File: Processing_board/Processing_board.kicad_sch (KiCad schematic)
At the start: 28 parts, among them J1 Conn_01x08_Pin, J2 Conn_01x08_Pin, J3 Conn_01x06_Pin, J4 Conn_01x03_Pin, J5 Conn_01x03_Pin, J6 Conn_01x02_Pin, J7 Conn_01x02_Pin, SW1 TL3305BF100QG, SW2 TL3305BF100QG, U1 STM32WBA63CIU6

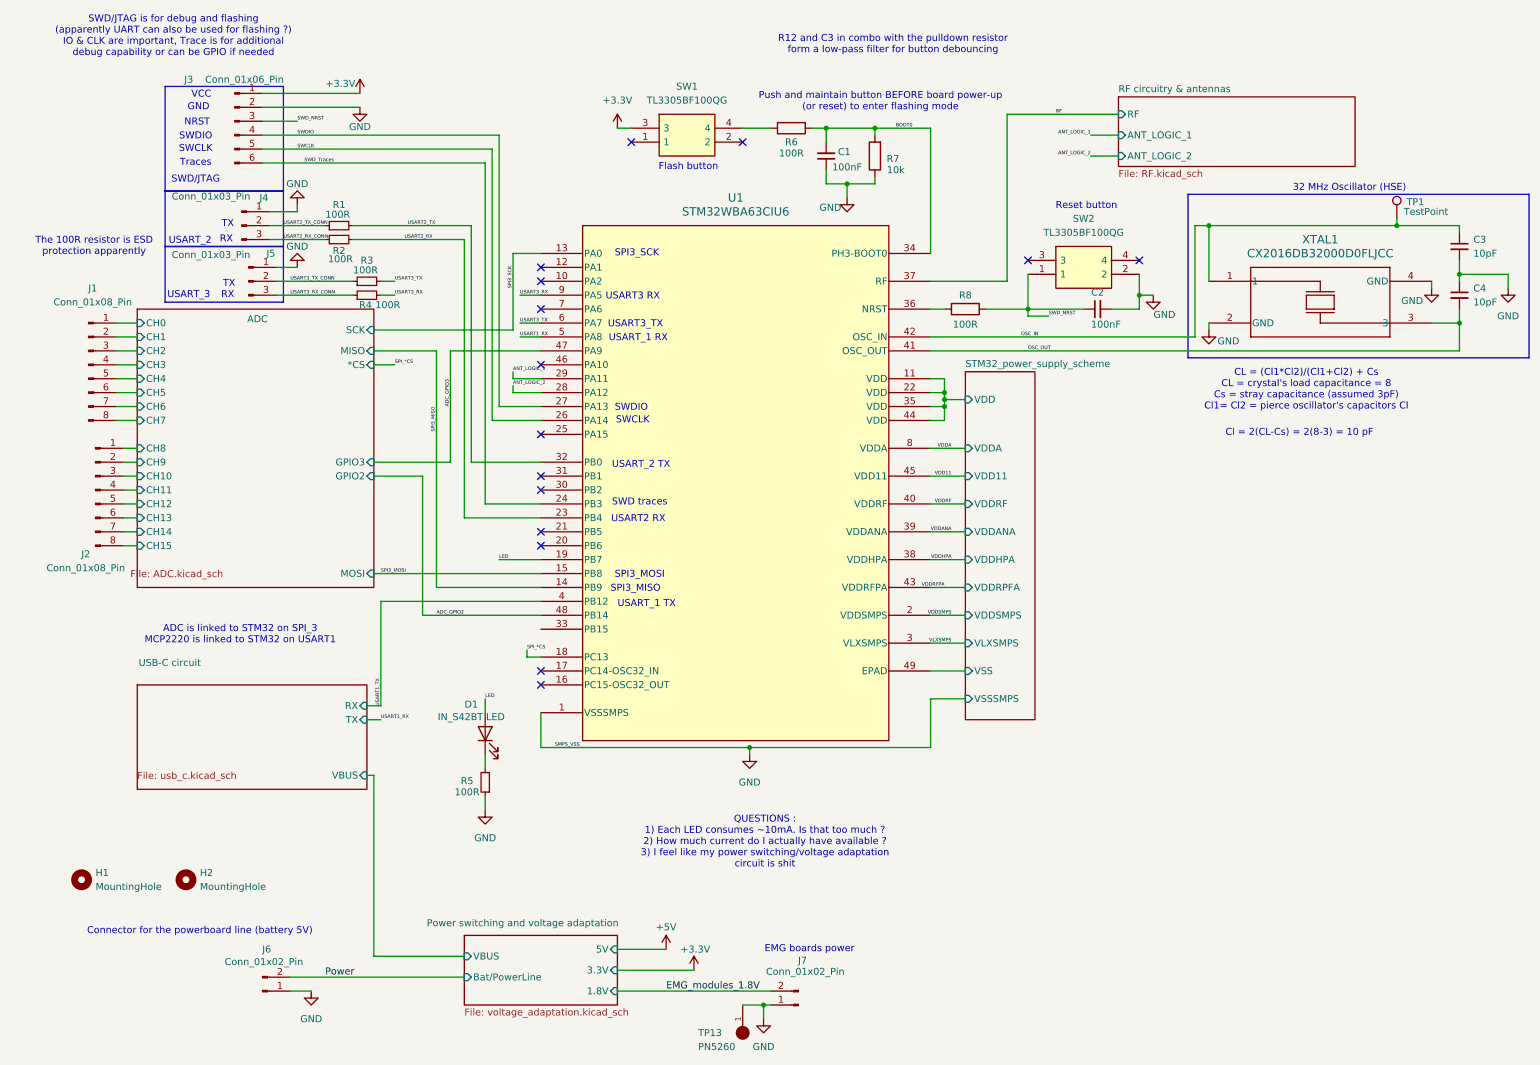
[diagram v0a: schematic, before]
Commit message: more cleanup
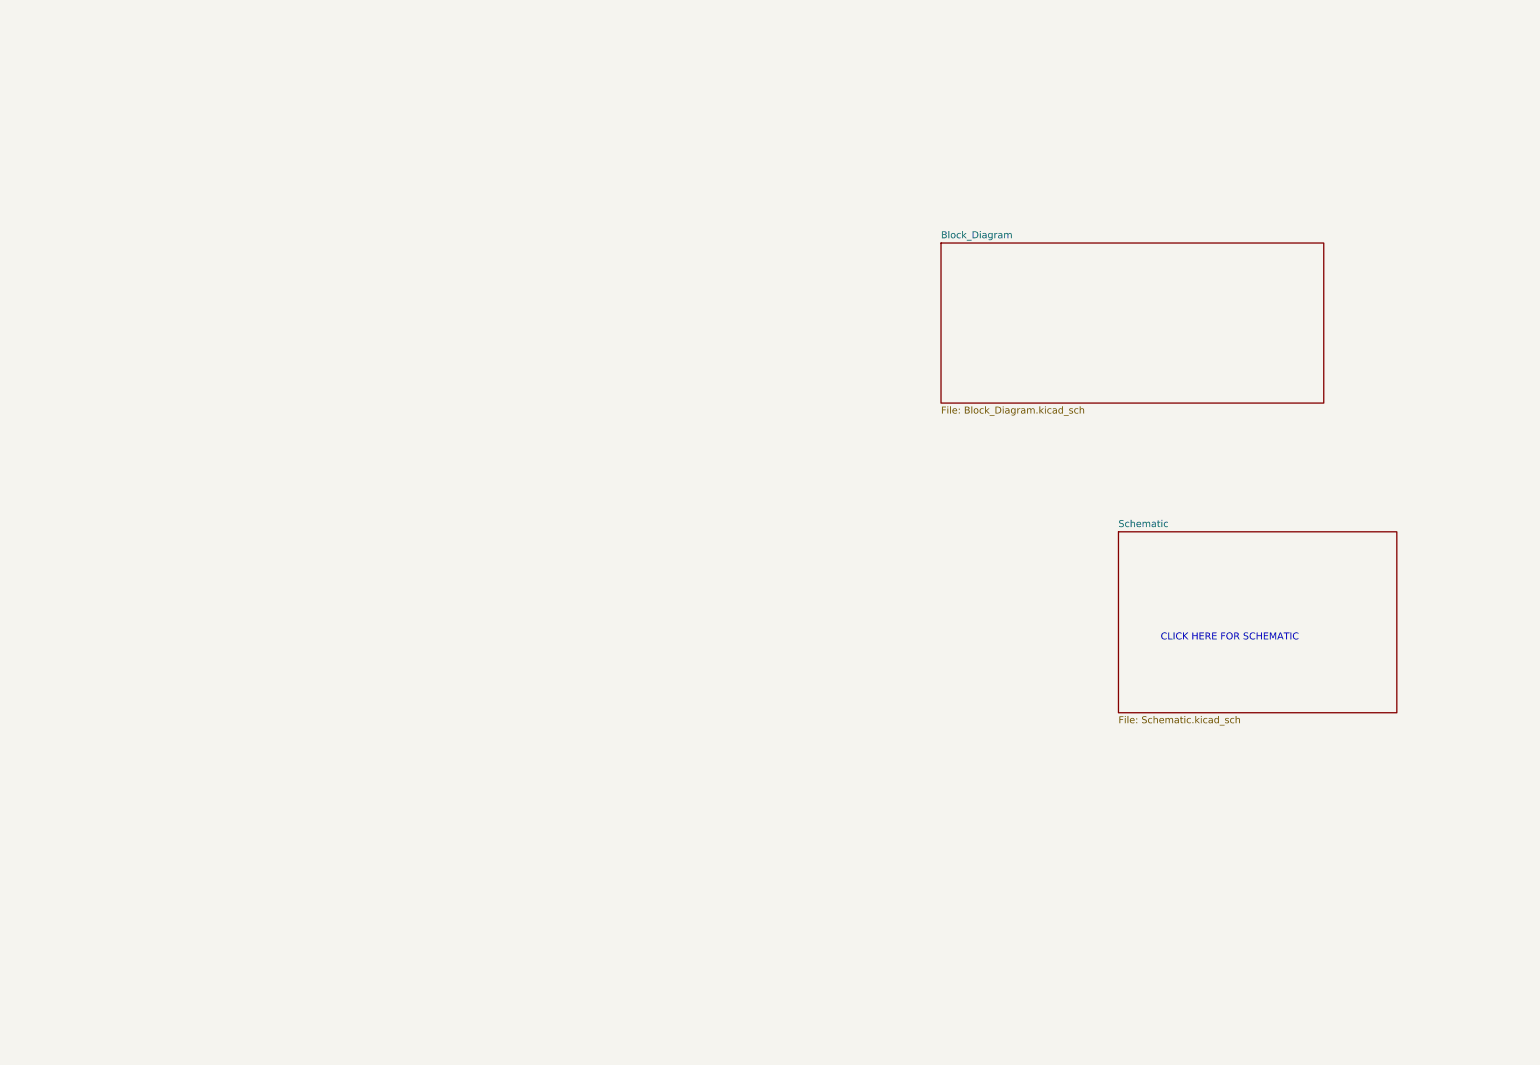
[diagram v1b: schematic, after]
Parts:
- removed C1, C2: 100nF, Capacitor_SMD:C_0402_1005Metric, symbol Device:C_Small
- removed C3, C4: 10pF, Capacitor_SMD:C_0603_1608Metric, symbol Device:C_Small
- removed D1: IN_S42BT LED, LED_SMD:LED_0402_1005Metric, symbol Device:LED
- removed H1, H2: MountingHole, MountingHole:MountingHole_2.2mm_M2, symbol Mechanical:MountingHole
- removed J1, J2: Conn_01x08_Pin, Connector_PinHeader_2.54mm:PinHeader_1x08_P2.54mm_Vertical_SMD_Pin1Left, symbol Connector:Conn_01x08_Pin
- removed J3: Conn_01x06_Pin, Connector_PinHeader_2.54mm:PinHeader_1x06_P2.54mm_Vertical_SMD_Pin1Left, symbol Connector:Conn_01x06_Pin
- removed J4, J5: Conn_01x03_Pin, Connector_PinHeader_2.54mm:PinHeader_1x03_P2.54mm_Vertical_SMD_Pin1Left, symbol Connector:Conn_01x03_Pin
- removed J6, J7: Conn_01x02_Pin, Connector_PinHeader_2.54mm:PinHeader_1x02_P2.54mm_Vertical_SMD_Pin1Left, symbol Connector:Conn_01x02_Pin
- removed R1, R2, R3, R4, R5: 100R, Resistor_SMD:R_0402_1005Metric, symbol Device:R_Small
- removed R6, R8: 100R, Resistor_SMD:R_0402_1005Metric, symbol Device:R
- removed R7: 10k, Resistor_SMD:R_0402_1005Metric, symbol Device:R
- removed SW1, SW2: TL3305BF100QG, TL3305BF100QG:TL3305BF160QG, symbol TL3305BF100QG:TL3305BF100QG
- removed TP1: TestPoint, TestPoint:TestPoint_Pad_D1.0mm, symbol Connector:TestPoint
- removed TP13: PN5260, PN5260:PN5260, symbol PN5260:5260
- removed U1: STM32WBA63CIU6, SMT32WBA63:UFQFPN-48_STM, symbol STM32WBA63CI:STM32WBA63CIU6
- removed XTAL1: CX2016DB32000D0FLJCC, CX2016DB32000D0FLJCC:xtal4_CX2016DB_AVX, symbol CX2016DB32000D0FLJCC:CX2016DB32000D0FLJCC
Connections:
- no-connect marks 15 -> 0
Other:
- removed sheet ADC
- removed sheet Power switching and voltage adaptation
- removed sheet RF circuitry & antennas
- removed sheet STM32_power_supply_scheme
- removed sheet USB-C circuit
- added sheet Block_Diagram (Block_Diagram.kicad_sch)
- added sheet Schematic (Schematic.kicad_sch)
- note added: "CLICK HERE FOR SCHEMATIC"
- note removed: "32 MHz Oscillator (HSE)"
- note removed: "ADC is linked to STM32 on SPI_3 MCP2220 is linked to STM32 on USART1"
- note removed: "CL = (Cl1*Cl2)/(Cl1+Cl2) + Cs CL = crystal's load capacitance = 8 Cs = stray capacitance (assumed 3pF) Cl1= Cl2 = pierce oscillator's capacitors Cl"
- note removed: "Cl = 2(CL-Cs) = 2(8-3) = 10 pF"
- note removed: "Connector for the powerboard line (battery 5V)"
- note removed: "EMG boards power"
- note removed: "Flash button"
- note removed: "GND"
- note removed: "NRST"
- note removed: "Push and maintain button BEFORE board power-up (or reset) to enter flashing mode"
- note removed: "QUESTIONS : 1) Each LED consumes ~10mA. Is that too much ? 2) How much current do I actually have available ? 3) I feel like my power switching/voltage adaptation circuit is shit"
- note removed: "R12 and C3 in combo with the pulldown resistor form a low-pass filter for button debouncing"
- note removed: "RX"
- note removed: "Reset button"
- note removed: "SPI3_MISO"
- note removed: "SPI3_MOSI"
- note removed: "SPI3_SCK"
- note removed: "SWCLK"
- note removed: "SWD traces"
- note removed: "SWD/JTAG"
- note removed: "SWD/JTAG is for debug and flashing (apparently UART can also be used for flashing ?) IO & CLK are important, Trace is for additional debug capability or can be GPIO if needed"
- note removed: "SWDIO"
- note removed: "TX"
- note removed: "The 100R resistor is ESD protection apparently"
- note removed: "Traces"
- note removed: "USART2 RX"
- note removed: "USART3 RX"
- note removed: "USART3_TX"
- note removed: "USART_1 RX"
- note removed: "USART_1 TX"
- note removed: "USART_2"
- note removed: "USART_2 TX"
- note removed: "USART_3"
- note removed: "VCC"
